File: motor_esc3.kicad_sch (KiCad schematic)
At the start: 14 parts, among them J10 SolderWirePad_1x01_SMD_3x6mm, J8 SolderWirePad_1x01_SMD_3x6mm, J9 SolderWirePad_1x01_SMD_3x6mm, U6 MCF8316A

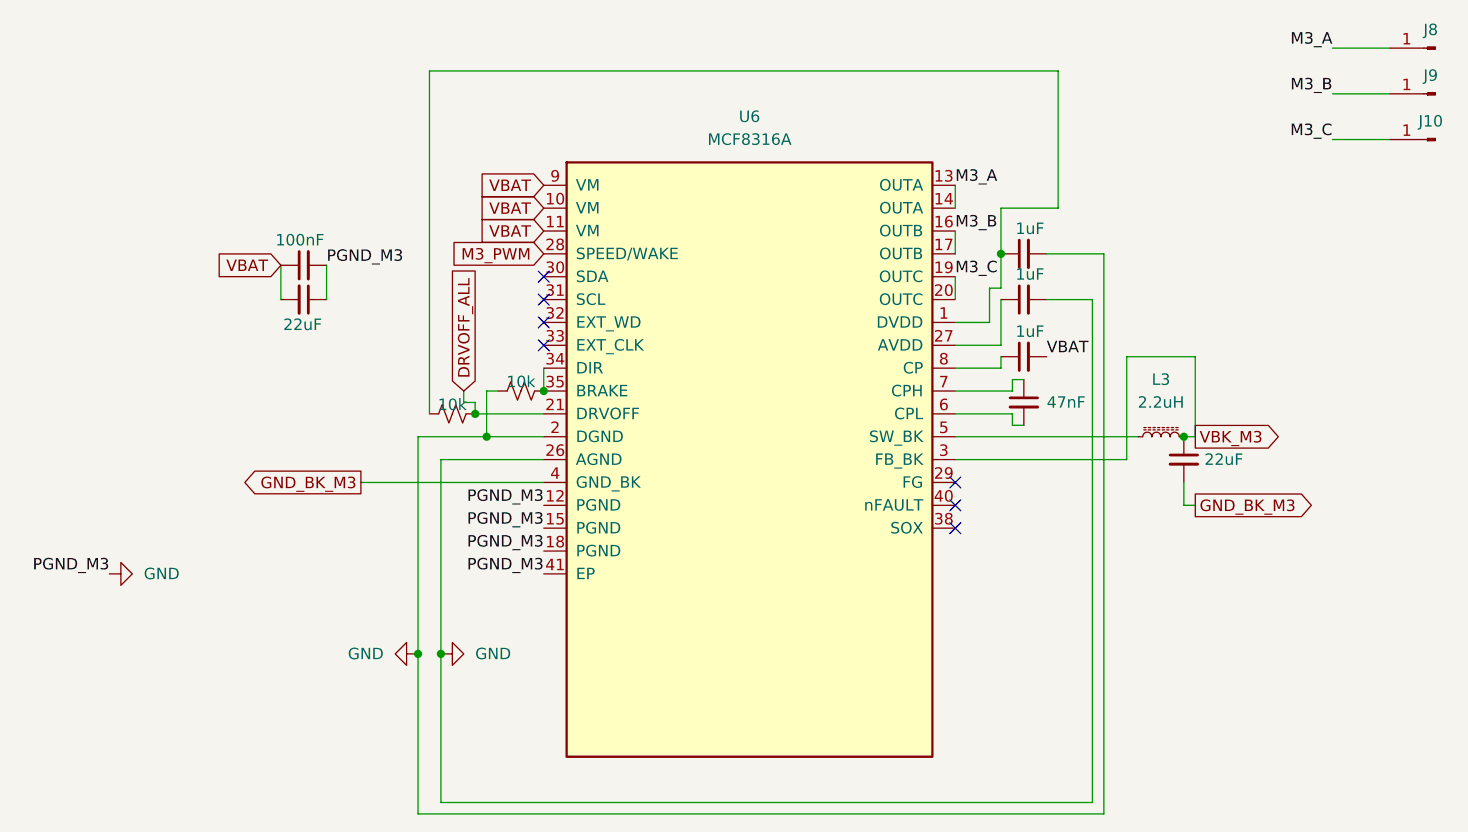
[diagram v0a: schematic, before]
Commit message: done?
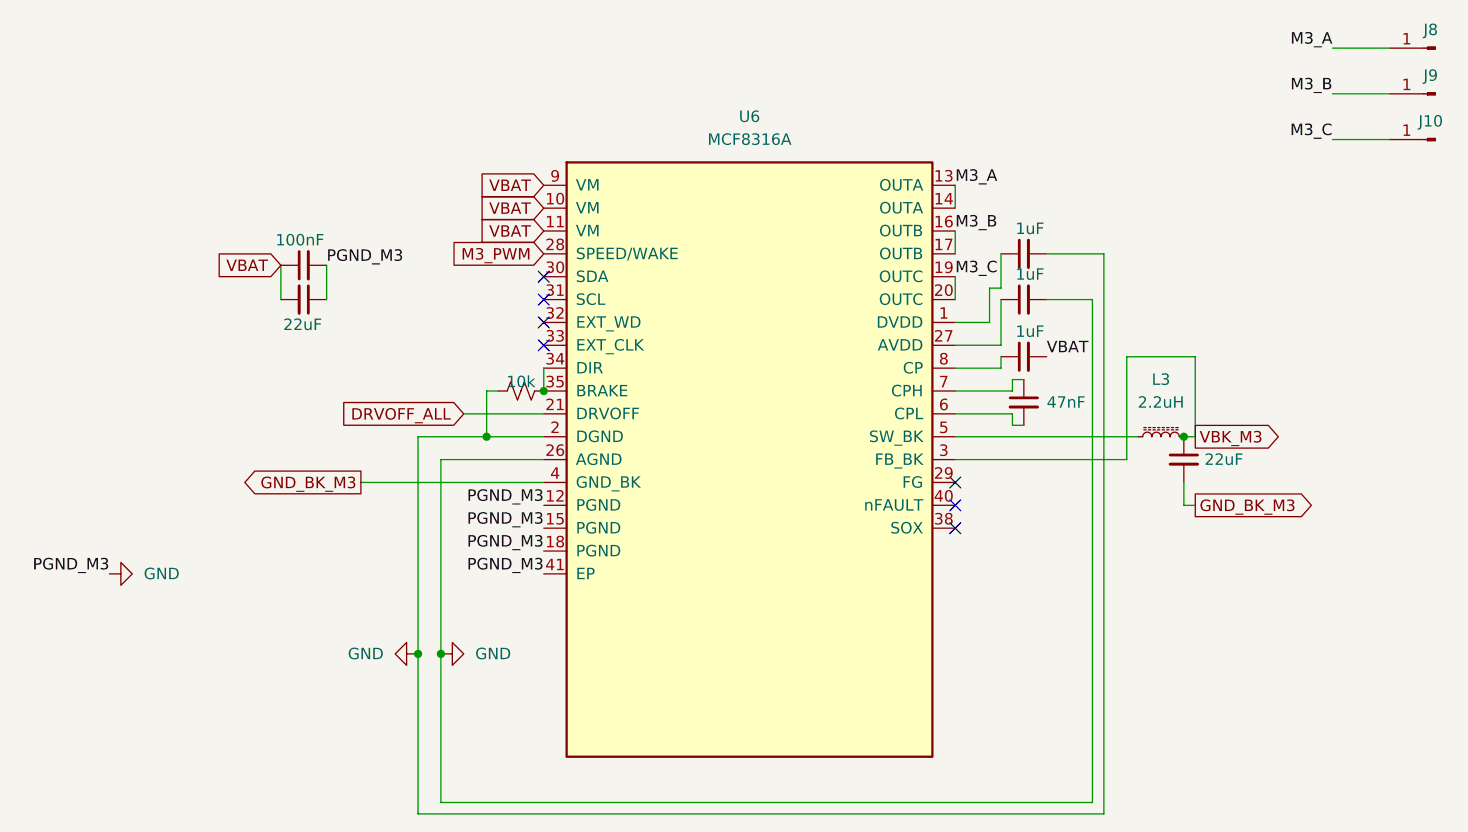
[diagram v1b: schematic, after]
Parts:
- removed R10: 10k, Resistor_SMD:R_0603_1608Metric_Pad0.98x0.95mm_HandSolder, symbol Device:R_Small_US
- R12: footprint Resistor_SMD:R_0603_1608Metric_Pad0.98x0.95mm_HandSolder -> Resistor_SMD:R_0402_1005Metric_Pad0.72x0.64mm_HandSolder
